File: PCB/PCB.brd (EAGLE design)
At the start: 41.7 x 50.2 mm, 17 parts, among them IC1 FT230XS, IC3 REG1117, X1 MINI-USB-32005-201

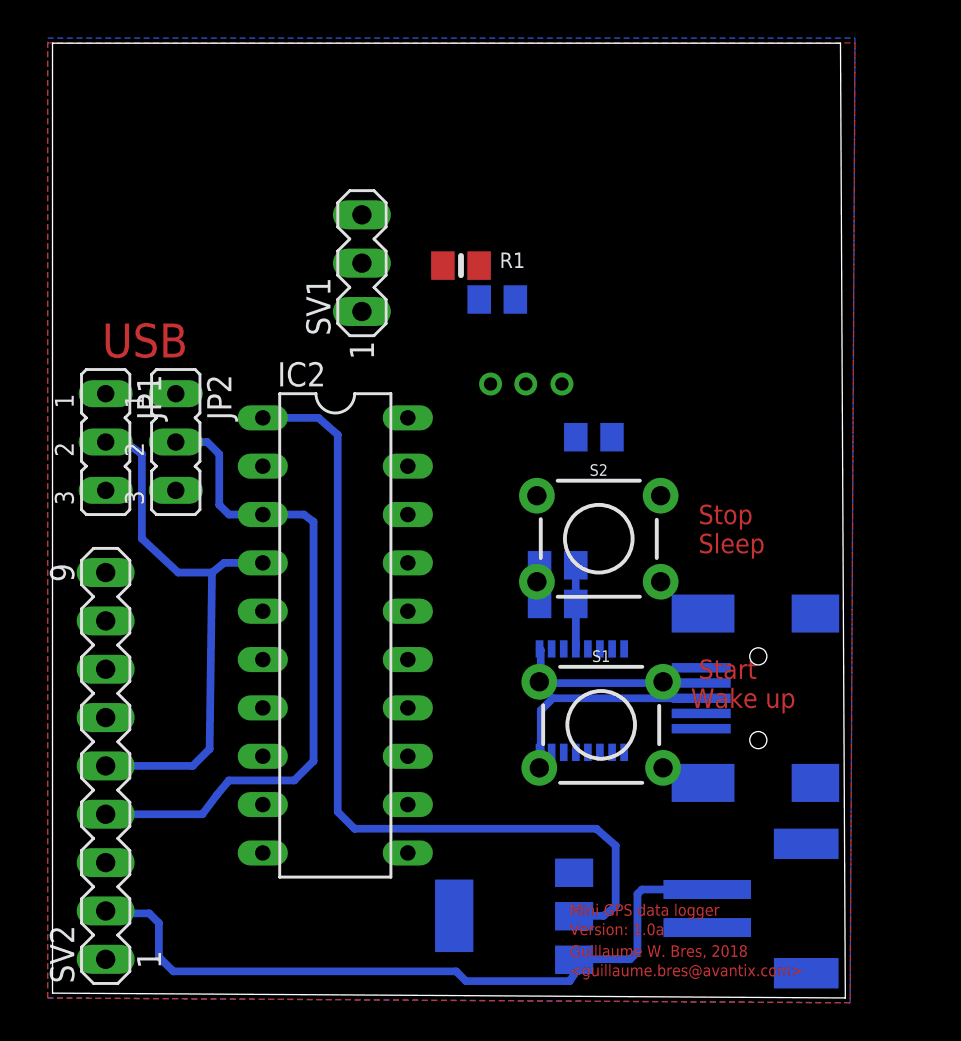
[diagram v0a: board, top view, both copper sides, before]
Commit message: v1.0 almost done
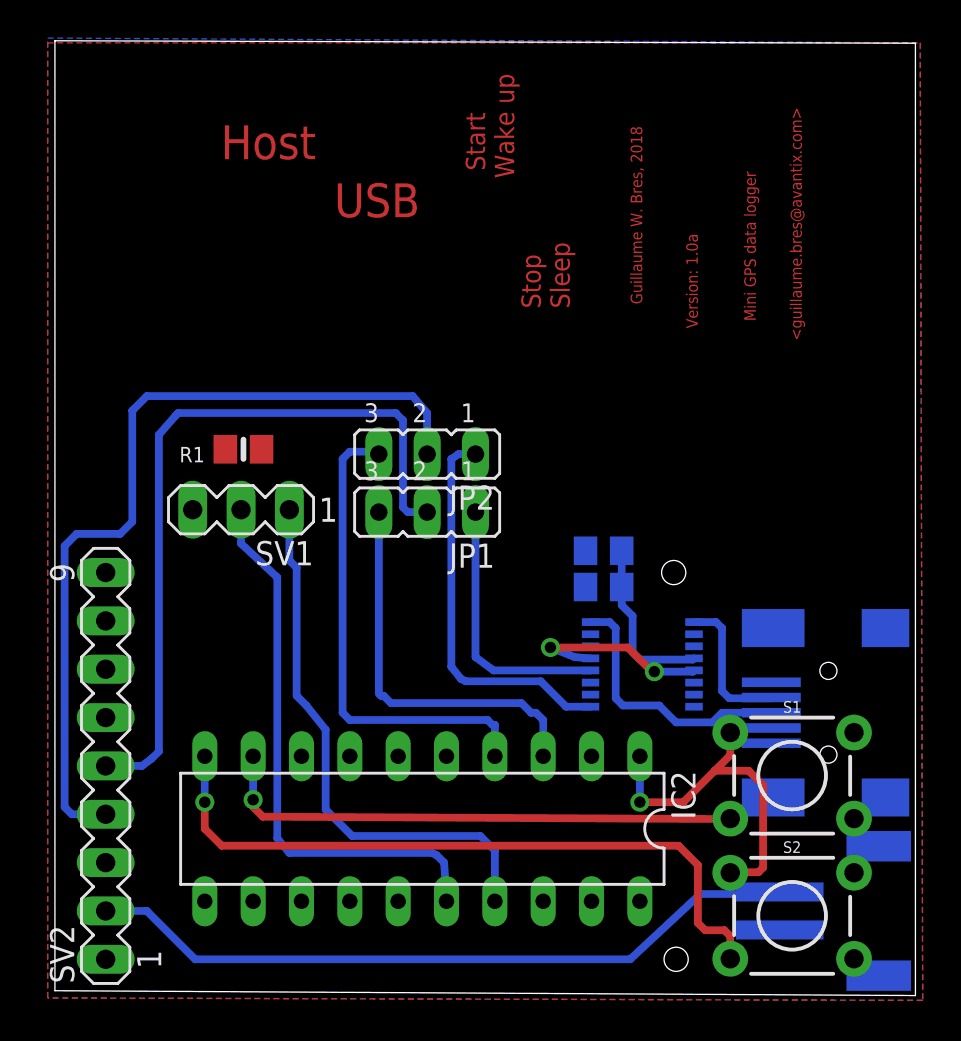
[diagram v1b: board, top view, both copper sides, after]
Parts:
- removed C4, C5: 22pF, microbuilder:0805-NO
- removed IC3: REG1117, burr-brown:SOT223
- removed QF1: 16M20AUM1, crystal:UM1
- moved S2 22.3 mm to (37.8, 4.06)
- moved JP1 17.3 mm to (18.7, 25.3), turned to 180 degrees
- moved R1 15.0 mm to (9.02, 28.6), turned to 180 degrees
- moved SV1 14.4 mm to (8.89, 25.4), turned to 180 degrees
- moved JP2 13.2 mm to (18.7, 28.3), turned to 180 degrees
- moved IC2 11.1 mm to (18.4, 8.64), turned to 180 degrees
- moved S1 10.4 mm to (37.8, 11.4)
- moved J1 3.81 mm to (40.9, 4.32)
- moved X1 3.76 mm to (39.8, 14.7)
- moved IC1 3.70 mm to (30.0, 17.3), turned to 180 degrees
- moved C3 3.69 mm to (27.9, 23.2)
- moved C2 2.67 mm to (27.9, 21.3)
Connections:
- removed net XIN: C4.2, QF1.1
- removed net XOUT: C5.1, QF1.3
- new net SW1: IC2.9, S1.3
- new net SW2: IC2.10, S2.3
- net 3.3V: now also S1.1, S2.1, SV2.9; no longer IC3.2
- net GND: no longer C4.1, C5.2, IC3.1
- net RX: no longer IC2.3
- net TX: no longer IC2.4
- net UC_RX: now also IC2.3
- net UC_TX: now also IC2.4
- net VBAT: no longer IC3.3
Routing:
- net SW2: track 0.00 -> 36.7 mm, vias 0 -> 1
- net RESET: track 0.00 -> 29.4 mm
- net TEST: track 0.00 -> 28.9 mm
- net SW1: track 0.00 -> 28.0 mm, vias 0 -> 1
- net 3.3V: track 44.9 -> 18.4 mm, vias 0 -> 1
- net UC_TX: track 0.00 -> 25.4 mm
- net UC_RX: track 0.00 -> 20.6 mm
- net FTDI_TX: track 0.00 -> 20.5 mm
- net FTDI_RX: track 0.00 -> 13.9 mm
- net GND: track 0.00 -> 10.9 mm, vias 0 -> 2
- net TX: track 28.9 -> 39.2 mm
- net RX: track 35.3 -> 44.3 mm
- net 5V: track 4.40 -> 8.98 mm
- net USB_DP: track 10.9 -> 14.0 mm
- net USB_DM: track 9.90 -> 7.67 mm
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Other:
- board size 41.7 x 50.2 mm -> 45.2 x 50.2 mm
- board text added: "Host"
